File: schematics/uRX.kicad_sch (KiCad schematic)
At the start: 89 parts, among them J1 RF_In, J3 AudioJack2_Ground, J4 +5Vfiltered, J5 +5V, J6 RF_In, J7 +3.3Vfiltered, P1 USB_C_Plug_USB2.0, U1 CBT3253, U11 IP2326, U2 LM4562, U3 ESP32-DEVKIT, U4 Si5351A-B-GT, U5 OPA2690, U6 Si4732-A10, U7 PCM1808PWR, U8 LM4040-2.5, U9 PCM1808PWR, Y1 25MHz, Y2 32768kHz

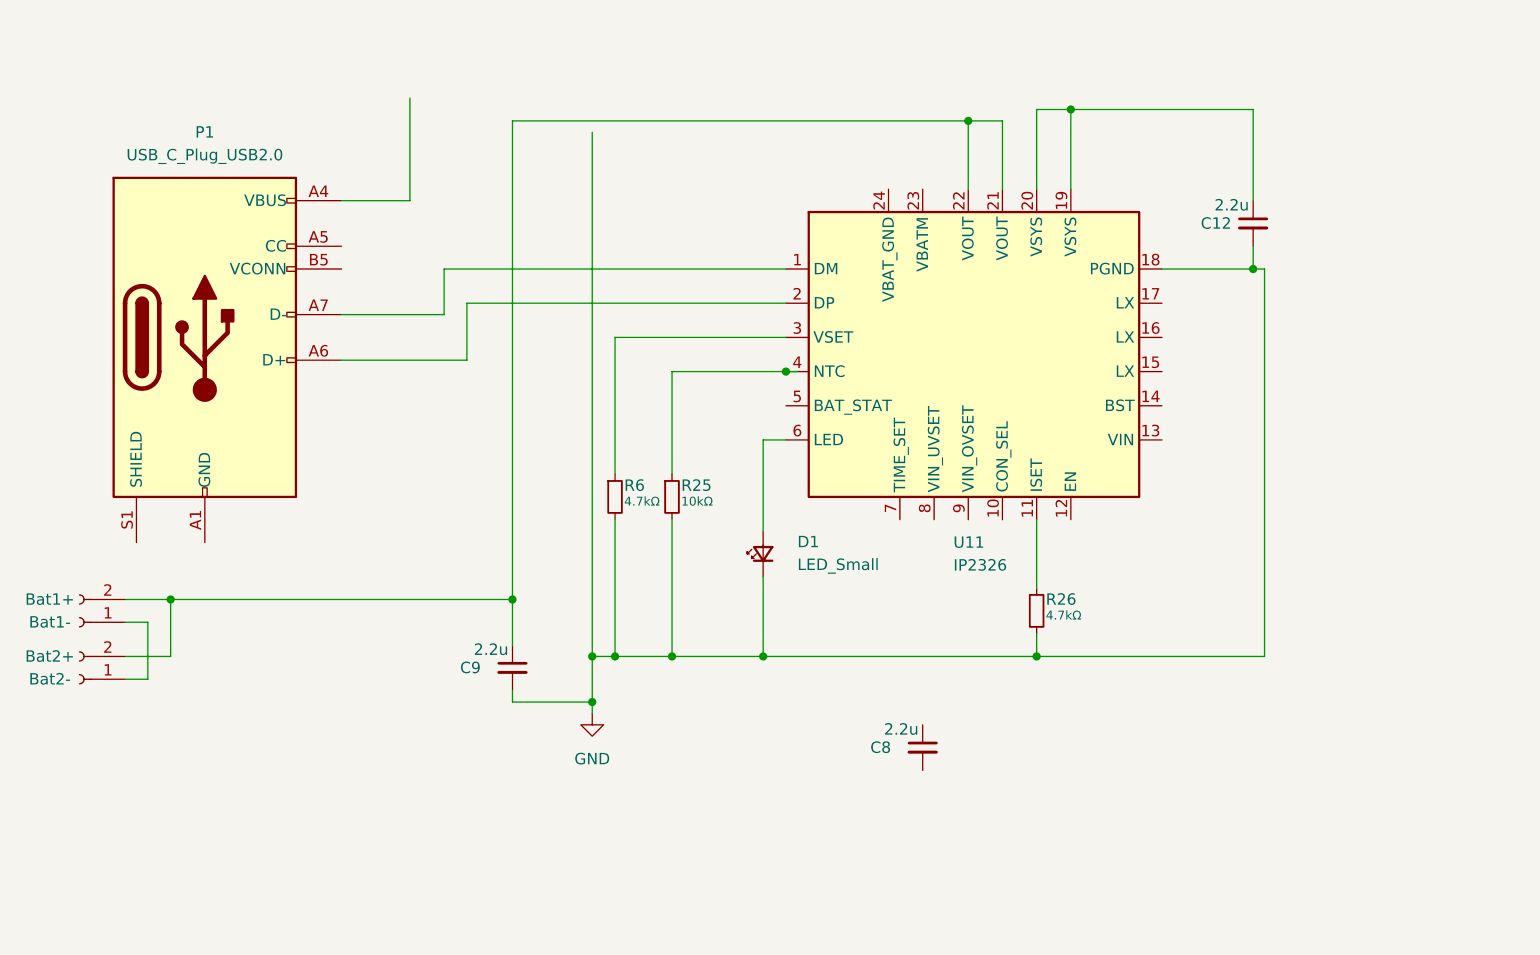
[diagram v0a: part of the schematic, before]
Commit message: finalize power circuit
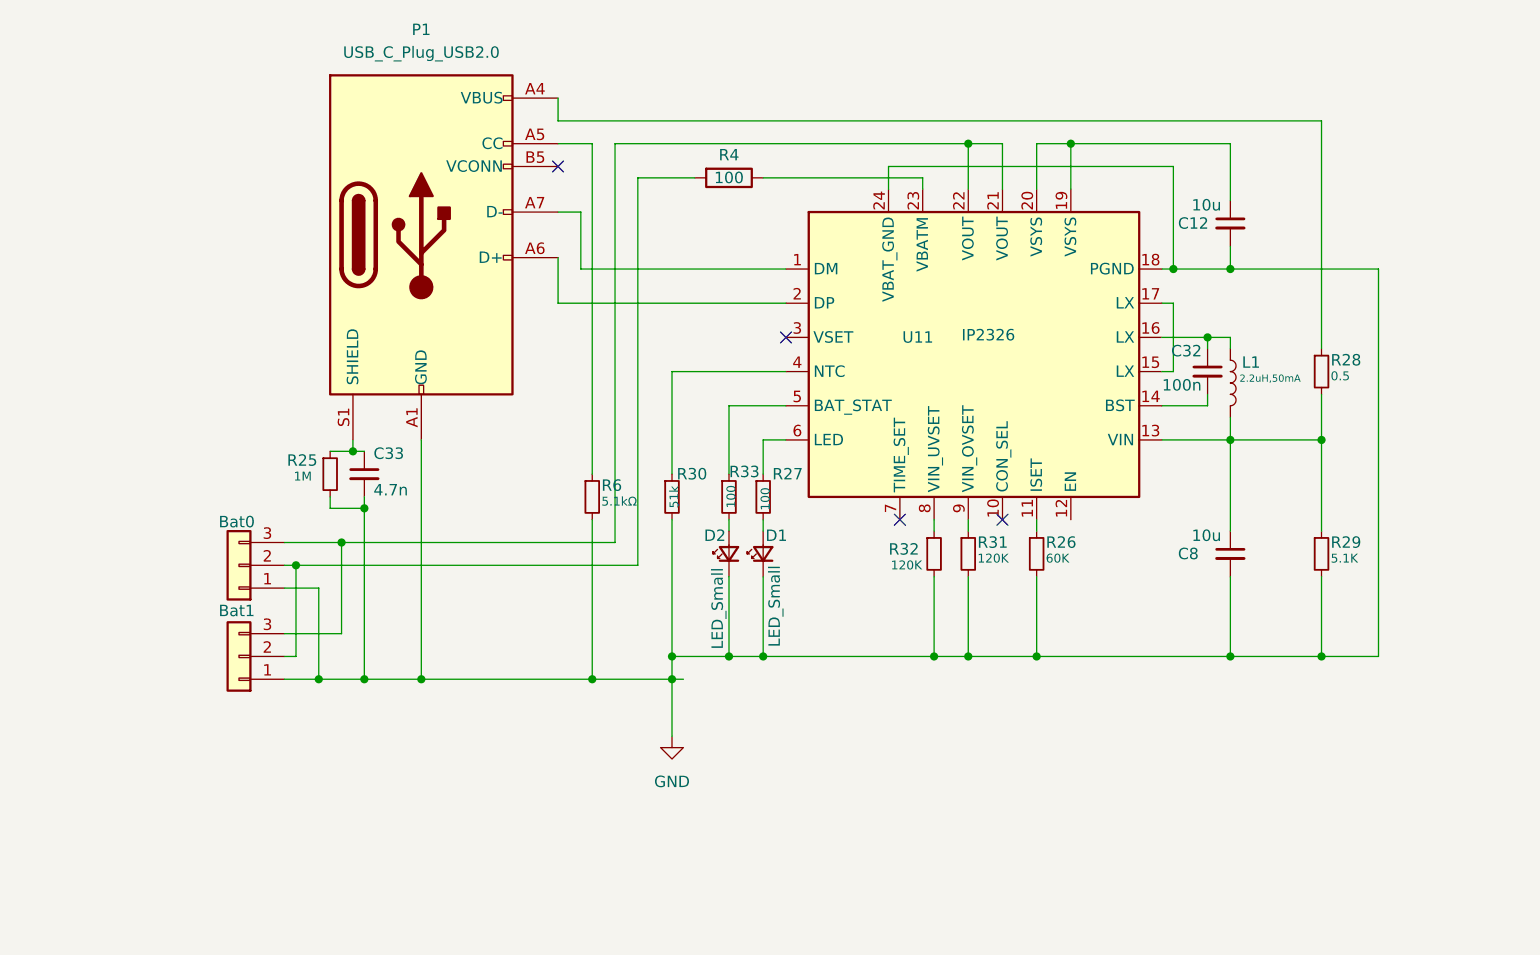
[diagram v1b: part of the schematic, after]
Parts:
- removed Bat1+: Bat1-, JST-XH, symbol Connector:Conn_01x02_Socket
- removed Bat2+: Bat2-, JST-XH, symbol Connector:Conn_01x02_Socket
- removed C9: 2.2u, Capacitor_SMD:C_0603_1608Metric, symbol Device:C_Small
- added Bat0, Bat1: JST-XH, symbol Connector_Generic:Conn_01x03
- added C32: 100n, Capacitor_SMD:C_0603_1608Metric, symbol Device:C_Small
- added C33: 4.7n, Capacitor_SMD:C_0603_1608Metric, symbol Device:C_Small
- added D2: LED_Small, symbol Device:LED_Small
- added L1: 2.2uH,50mA, PCM_JLCPCB:L_0805, symbol PCM_JLCPCB-Inductors:1uH,50mA
- added R27, R33: 100, Resistor_SMD:R_0603_1608Metric, symbol Device:R_Small
- added R28: 0.5, Resistor_SMD:R_0603_1608Metric, symbol Device:R_Small
- added R29: 5.1K, Resistor_SMD:R_0603_1608Metric, symbol Device:R_Small
- added R30: 51k, Resistor_SMD:R_0603_1608Metric, symbol Device:R_Small
- added R31, R32: 120K, Resistor_SMD:R_0603_1608Metric, symbol Device:R_Small
- added R4: 100, Resistor_SMD:R_0603_1608Metric, symbol Device:R
- C12, C8: value 2.2u -> 10u
- R25: value 10kΩ -> 1M
- R26: value 4.7kΩ -> 60K
- R6: value 4.7kΩ -> 5.1kΩ
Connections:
- net GND: now also C8.2, P1.A1 (GND), P1.A12 (GND), P1.B1 (GND), P1.B12 (GND), U11.24 (VBAT_GND), Bat0.1 (Pin_1), Bat1.1 (Pin_1), C33.2, D2.1 (K), R29.2, R30.2, R31.2, R32.2
- net at P1.A4 (VBUS), P1.A9 (VBUS), P1.B4 (VBUS)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: now also R28.1
- net at P1.A5 (CC): now also R6.1
- net at P1.S1 (SHIELD): now also R25.1, C33.1
- net at U11.21 (VOUT), U11.22 (VOUT): now also Bat0.3 (Pin_3), Bat1.3 (Pin_3)
- net at D1.2 (A): now also R27.2; no longer U11.6 (LED)
- net at U11.3 (VSET): no longer R6.1
- net at U11.4 (NTC): now also R30.1; no longer R25.1
- net at U11.13 (VIN): now also C8.1, L1.2, R28.2, R29.1
- net at U11.14 (BST): now also C32.2
- net at U11.15 (LX): now also U11.17 (LX)
- net at U11.16 (LX): now also C32.1, L1.1
- net at U11.23 (VBATM): now also R4.1
- net at U11.25 (GND), U11.8 (VIN_UVSET): now also R32.1
- net at U11.5 (BAT_STAT): now also R33.1
- net at U11.9 (VIN_OVSET): now also R31.1
- new net: Bat0.2 (Pin_2), Bat1.2 (Pin_2), R4.2
- new net: R27.1, U11.6 (LED)
- new net: D2.2 (A), R33.2
- no-connect marks 15 -> 19
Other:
- moved on the sheet: C12, C8, P1, R26
